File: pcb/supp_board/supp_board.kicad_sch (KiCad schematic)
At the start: 19 parts, among them J1 Conn_01x03_Pin, J2 Conn_01x02_Pin, J3 Screw_Terminal_01x04, J4 Screw_Terminal_01x04, J5 Screw_Terminal_01x04, J6 Conn_01x08_Socket, J7 Conn_01x08_Socket, J8 Conn_01x08_Socket, J9 Conn_01x08_Socket, Q1 IRLZ44N, Q2 IRLZ44N, Q3 IRLZ44N, Q7 IRLZ44N, Q8 IRLZ44N, Q9 IRLZ44N

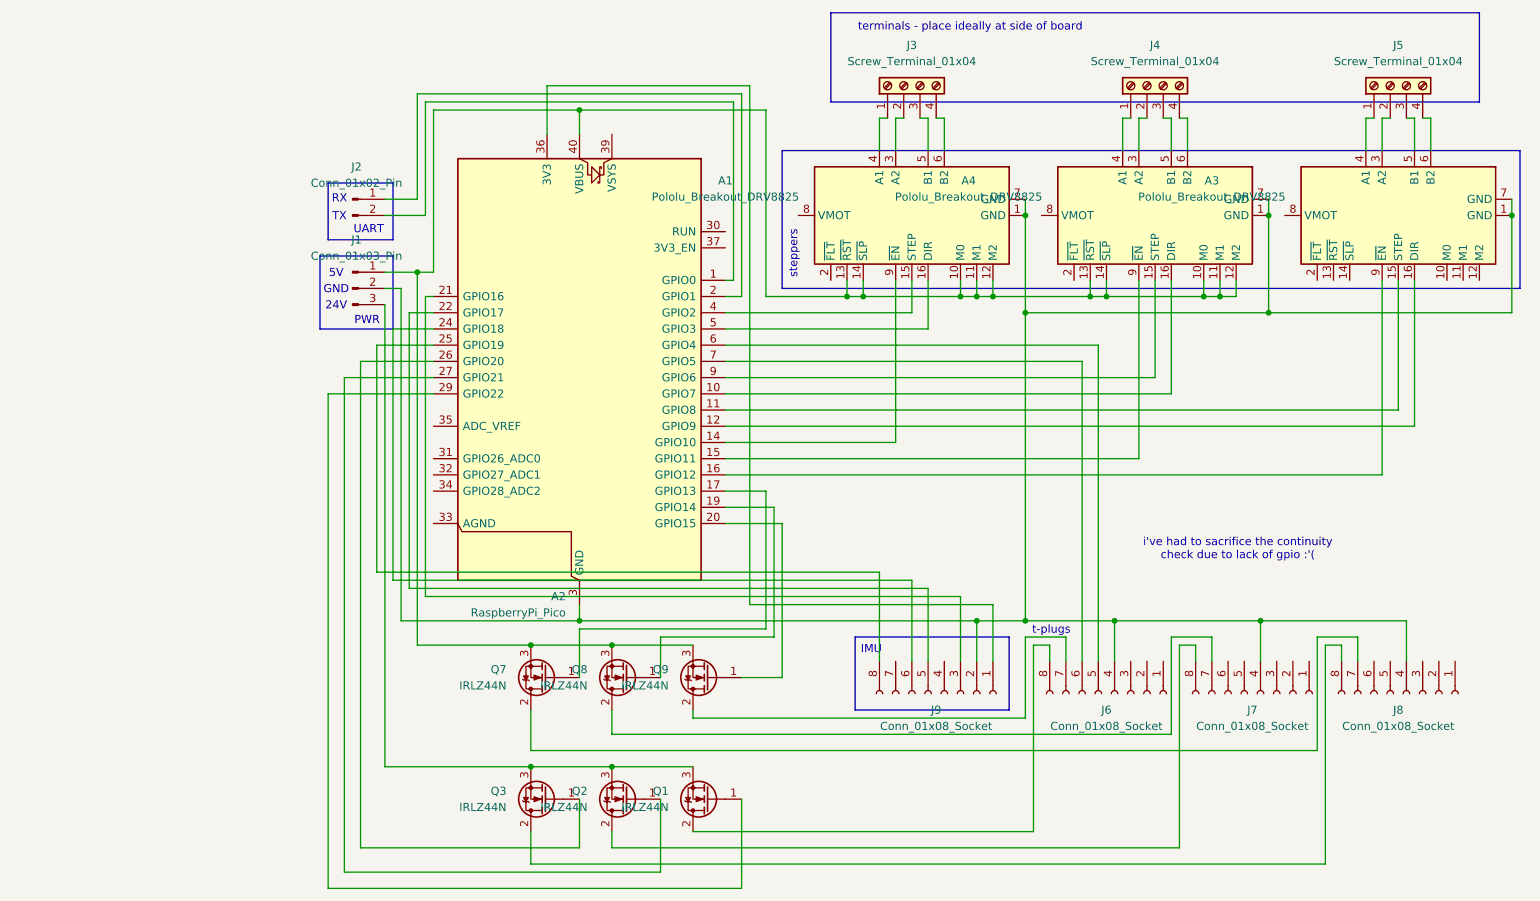
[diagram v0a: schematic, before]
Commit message: Add work from 2025-07-24 to 2025-07-26
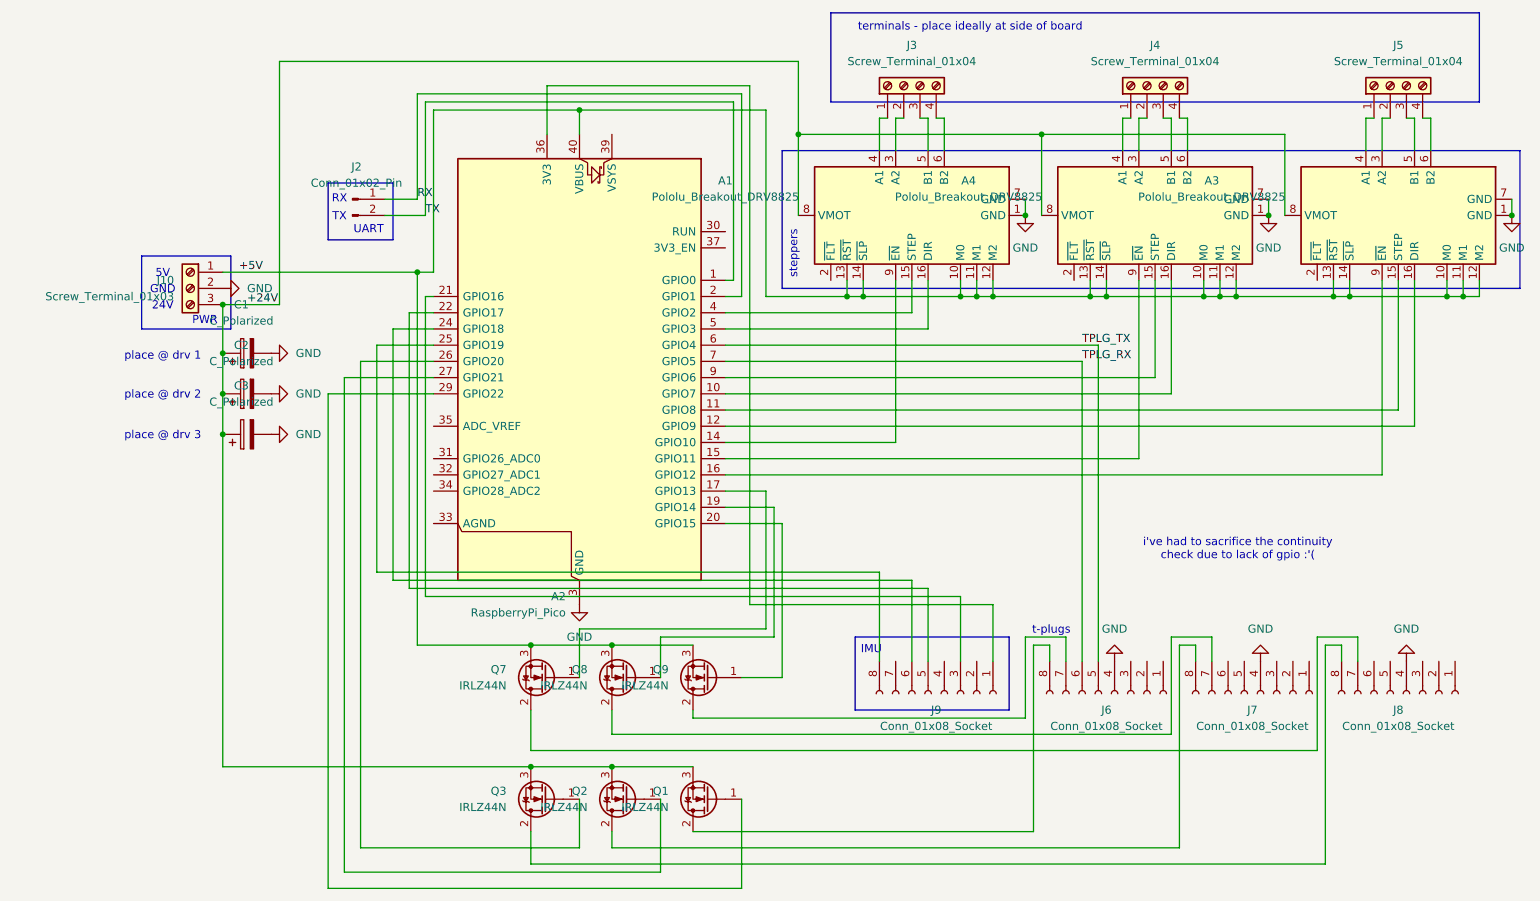
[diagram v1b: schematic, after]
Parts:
- removed J1: Conn_01x03_Pin, Connector_Wire:SolderWire-0.5sqmm_1x03_P4.6mm_D0.9mm_OD2.1mm, symbol Connector:Conn_01x03_Pin
- added C1, C2, C3: C_Polarized, Capacitor_THT:CP_Radial_D8.0mm_P3.50mm, symbol Device:C_Polarized
- added J10: Screw_Terminal_01x03, TerminalBlock:TerminalBlock_MaiXu_MX126-5.0-03P_1x03_P5.00mm, symbol Connector:Screw_Terminal_01x03
- J6, J7, J8, J9: footprint Connector_JST:JST_PH_S8B-PH-K_1x08_P2.00mm_Horizontal -> Connector_JST:JST_PH_B8B-PH-K_1x08_P2.00mm_Vertical
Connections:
- net TX: now reaches A2.1 (GPIO0), J2.2 (Pin_2)
- net GND: now reaches A1.1 (GND), A1.7 (GND), A2.13 (GND), A2.18 (GND), A2.23 (GND), A2.28 (GND), A2.3 (GND), A2.38 (GND), A2.8 (GND), A3.1 (GND), A3.7 (GND), A4.1 (GND), A4.7 (GND), J6.4 (Pin_4), J7.4 (Pin_4), J8.4 (Pin_4)
- net GND: now also C1.2, C2.2, C3.2, J10.2 (Pin_2); no longer J9.2 (Pin_2)
- net RX: now reaches A2.2 (GPIO1), J2.1 (Pin_1)
- net +5V: now reaches A1.10 (M0), A1.11 (M1), A1.12 (M2), A1.13 (~{RST}), A1.14 (~{SLP}), A2.40 (VBUS), A4.10 (M0), A4.11 (M1), A4.12 (M2), A4.13 (~{RST}), A4.14 (~{SLP}), Q7.3 (S), Q8.3 (S), Q9.3 (S)
- net +5V: now also A3.10 (M0), A3.11 (M1), A3.12 (M2), A3.13 (~{RST}), A3.14 (~{SLP}), J10.1 (Pin_1)
- net TPLG_TX: now reaches A2.6 (GPIO4), J6.5 (Pin_5)
- net TPLG_RX: now reaches A2.7 (GPIO5), J6.6 (Pin_6)
- net +24V: now reaches Q1.3 (S), Q2.3 (S), Q3.3 (S)
- net +24V: now also A1.8 (VMOT), A3.8 (VMOT), A4.8 (VMOT), C1.1, C2.1, C3.1, J10.3 (Pin_3)
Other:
- note added: "place @ drv 1"
- note added: "place @ drv 2"
- note added: "place @ drv 3"
